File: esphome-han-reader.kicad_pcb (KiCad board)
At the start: 2 copper layers, 45 x 43.5 mm, 16 parts, among them J1 RJ12, J2 ProgammingPins, Q1 BC817W, SW1 ResetBtn, SW2 FlashBtn, U1 ESP-07, U2 LD1117S33CTR_SOT223

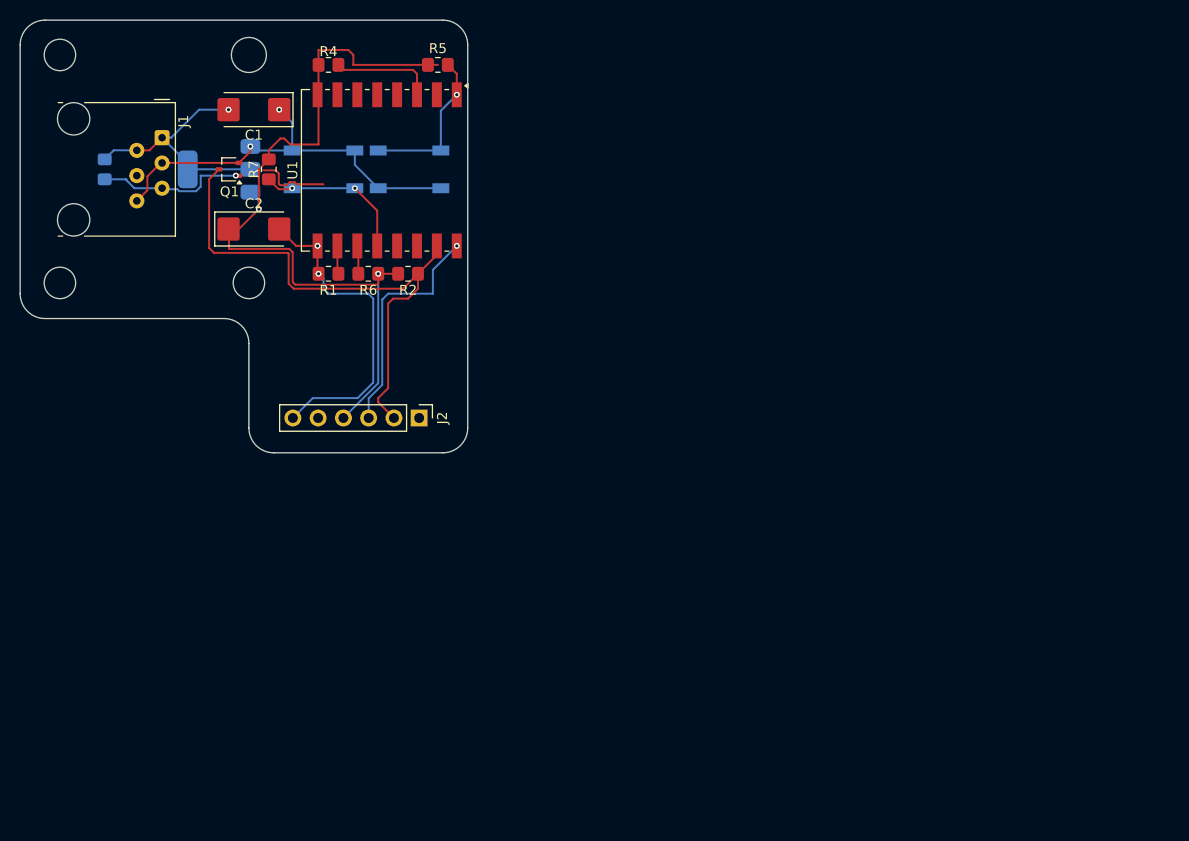
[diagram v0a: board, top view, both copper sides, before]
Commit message: feat: Final Rev??
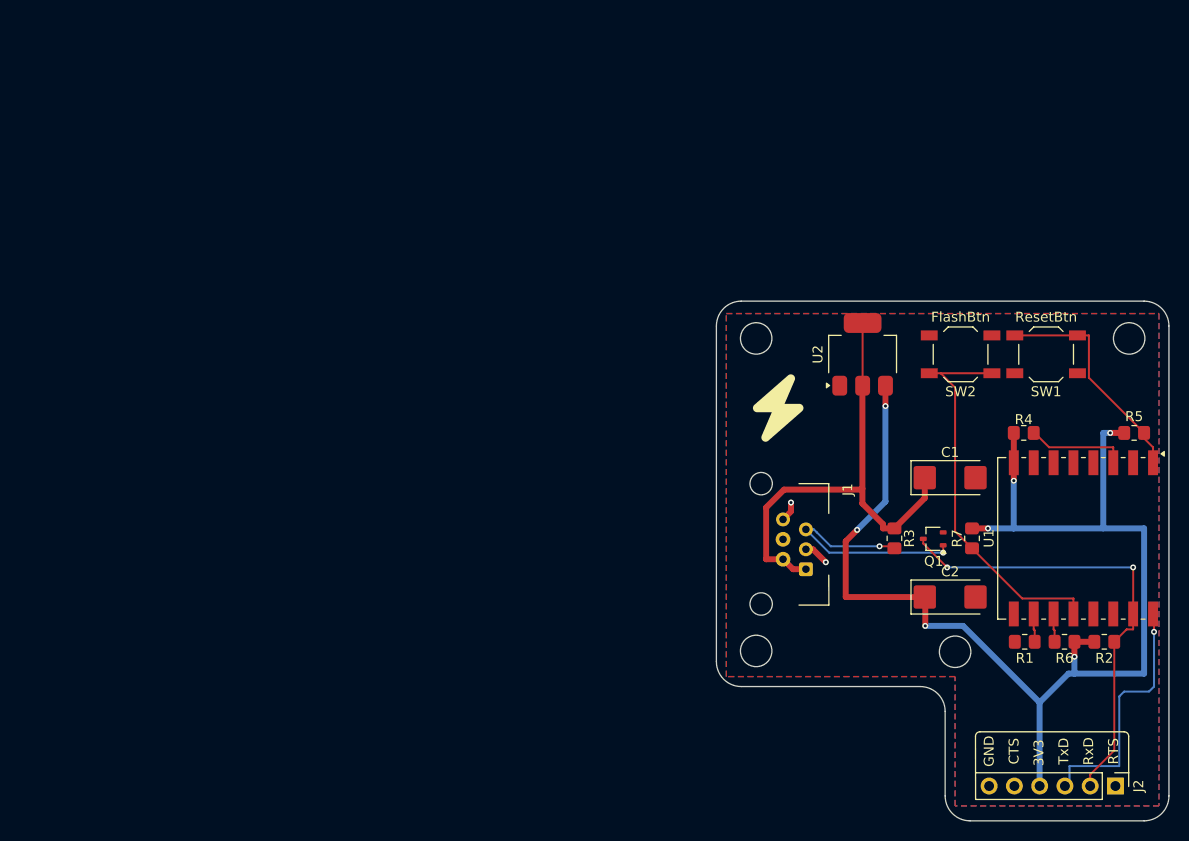
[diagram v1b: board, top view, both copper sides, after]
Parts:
- J1: footprint Connector_RJ:RJ12_Amphenol_54601-x06_Horizontal -> Connector_RJ:RJ12_DS1133-S60BPX
- J2: footprint Connector_PinHeader_2.54mm:PinHeader_1x06_P2.54mm_Vertical -> Connector_PinHeader_2.54mm:PinHeader_1x06_P2.54mm_Vertical_NoSilkscreen
- R2: value R2 -> 10K
- R3, SW1, SW2, U2: moved to F.Cu
- R5: value R5 -> 10K
- moved R3 87.6 mm to (144.9, 97.1)
- moved Q1 80.0 mm to (148.8, 97.2)
- moved R7 79.8 mm to (152.7, 97.1)
- moved C1 79.2 mm to (150.5, 91.0), turned to 0 degrees
- moved C2 79.2 mm to (150.5, 103.0)
- moved J2 79.2 mm to (167.1, 122.0)
- moved R1 79.2 mm to (158.0, 107.5)
- moved R2 79.2 mm to (166.0, 107.5), turned to 180 degrees
- moved R5 79.2 mm to (169.0, 86.5)
- moved R6 79.2 mm to (162.0, 107.5)
- moved U1 79.2 mm to (166.0, 97.1)
- moved R4 79.1 mm to (157.9, 86.5)
- moved J1 72.7 mm to (131.6, 97.3), turned to 0 degrees
- moved U2 67.3 mm to (141.7, 78.6), turned to 90 degrees
- moved SW2 66.7 mm to (151.6, 78.6), turned to 180 degrees
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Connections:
- C1 pad 1: GND -> +5V
- C1 pad 2: +5V -> GND
- R2 pad 1: +3V3 -> ESP-RX
- R2 pad 2: ESP-RX -> +3V3
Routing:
- net GND: track 74.4 -> 4.75 mm, vias 4 -> 2
- net +3V3: track 80.1 -> 127.1 mm, vias 2 -> 7
- net GPIO 0: track 16.0 -> 39.0 mm, vias 2 -> 0
- net +5V: track 27.1 -> 49.1 mm, vias 2 -> 0
- net Net-(Q1-B): track 15.0 -> 25.8 mm, vias 1 -> 2
- net ESP-RX: track 54.7 -> 46.7 mm, vias 0 -> 2
- net (no net): track 7.46 -> 0.00 mm
- net RESET: track 16.1 -> 22.9 mm, vias 1 -> 0
- net ESP-TX: track 23.6 -> 25.4 mm
- added copper zone on B.Cu, net GND
- added copper zone on F.Cu, net GND
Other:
- board size 45 x 43.5 mm -> 45.5 x 52.2 mm
- board text added: "3V3"
- board text added: "CTS"
- board text added: "GND"
- board text added: "JLCJLCJLCJLC"
- board text added: "LCHoldings/esphome-han-reader"
- board text added: "RTS"
- board text added: "RxD"
- board text added: "TxD"
